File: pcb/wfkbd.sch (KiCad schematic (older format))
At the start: 124 parts, among them J1 MJ-4PP-9, P1 LED, SW1 KEY, SW10 KEY, SW11 KEY, SW12 KEY, SW13 KEY, SW14 KEY, SW15 KEY, SW16 KEY, SW17 KEY, SW18 KEY, SW19 KEY, SW2 KEY, SW20 KEY, SW21 KEY, SW22 KEY, SW23 KEY, SW24 KEY, SW25 KEY, SW26 KEY, SW27 KEY, SW28 KEY, SW29 KEY, SW3 KEY, SW30 KEY, SW31 KEY, SW32 KEY, SW33 KEY, SW34 KEY, SW35 KEY, SW4 KEY, SW5 KEY, SW6 KEY, SW7 KEY, SW8 KEY, SW9 KEY, U1 ProMicro

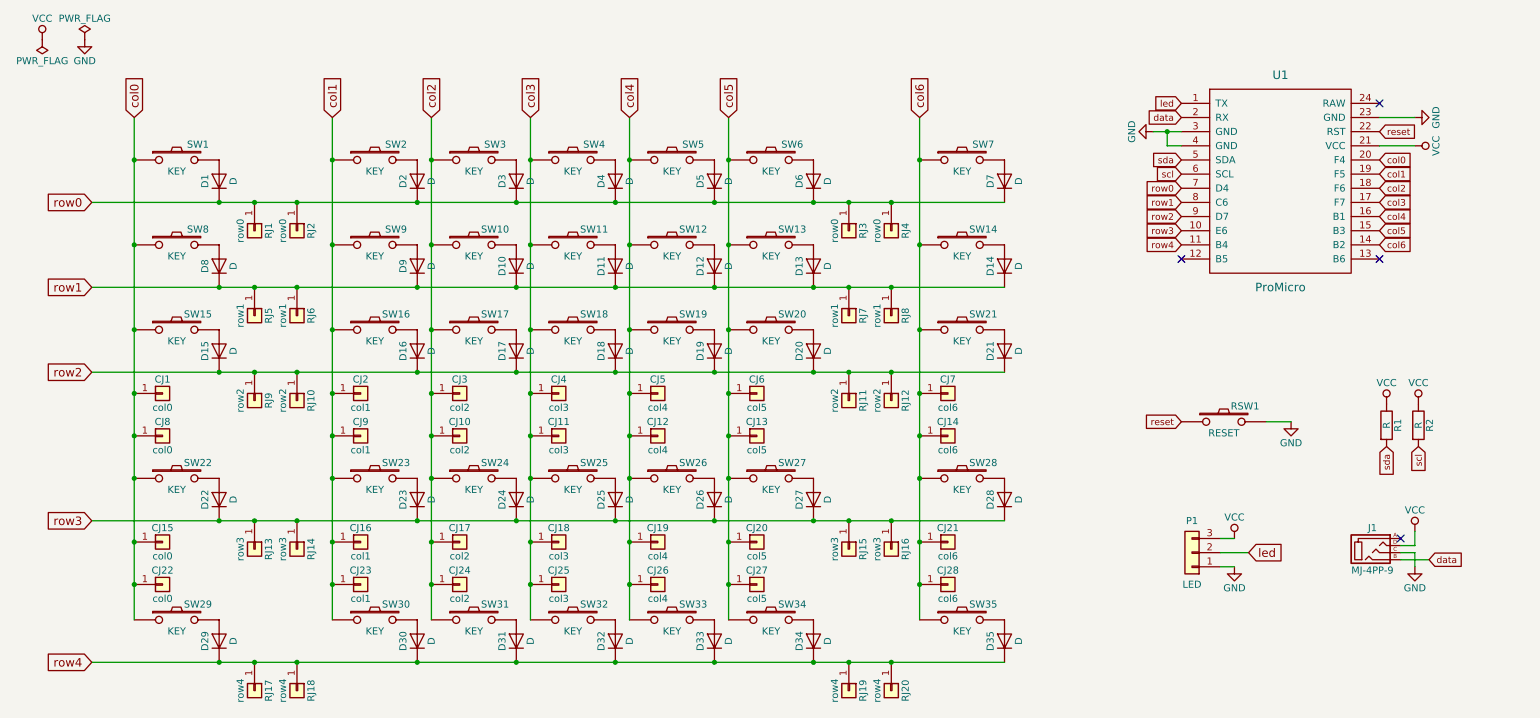
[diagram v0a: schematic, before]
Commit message: Add pcbnew files
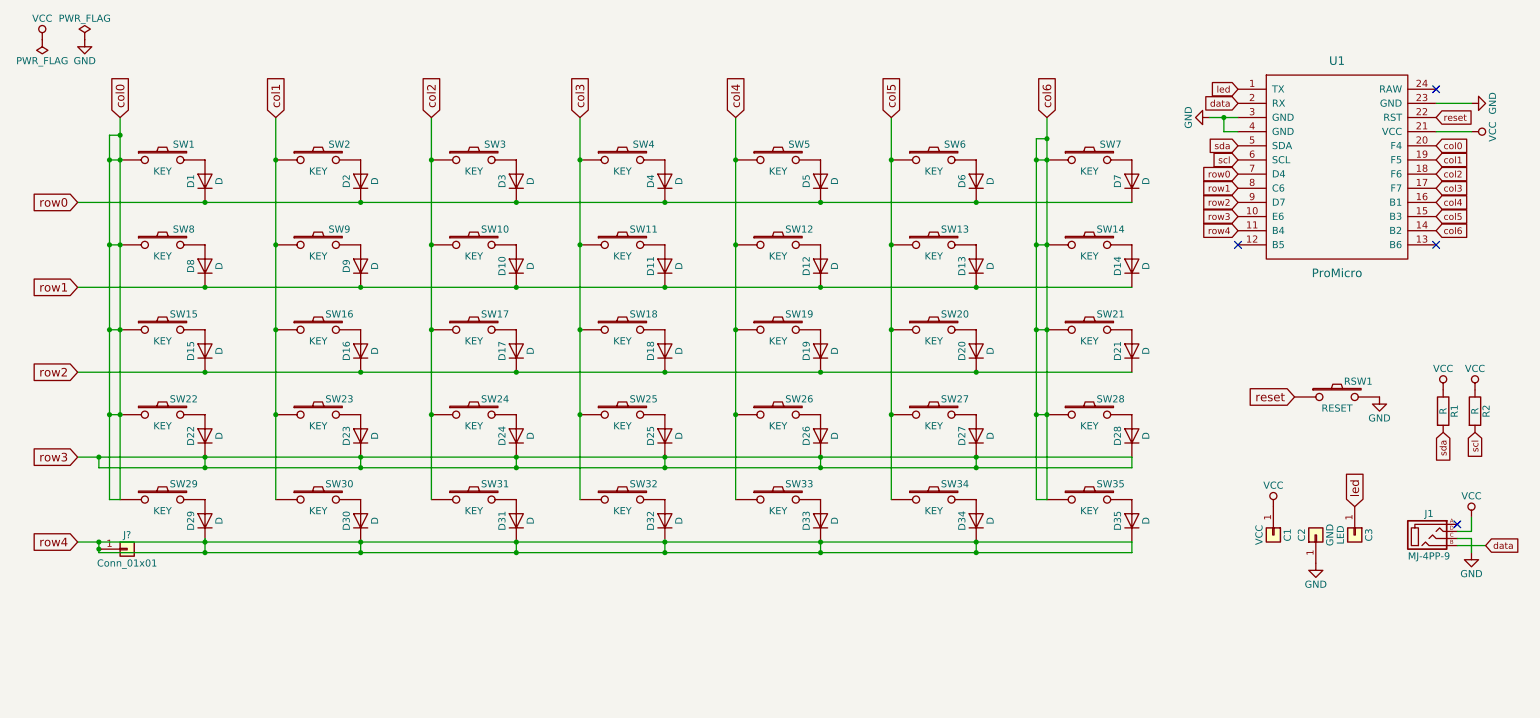
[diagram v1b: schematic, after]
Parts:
- removed CJ1, CJ15, CJ22, CJ8: col0, kbd:1pin_conn, symbol Conn_01x01
- removed CJ10, CJ17, CJ24, CJ3: col2, kbd:1pin_conn, symbol Conn_01x01
- removed CJ11, CJ18, CJ25, CJ4: col3, kbd:1pin_conn, symbol Conn_01x01
- removed CJ12, CJ19, CJ26, CJ5: col4, kbd:1pin_conn, symbol Conn_01x01
- removed CJ13, CJ20, CJ27, CJ6: col5, kbd:1pin_conn, symbol Conn_01x01
- removed CJ14, CJ21, CJ28, CJ7: col6, kbd:1pin_conn, symbol Conn_01x01
- removed CJ16, CJ2, CJ23, CJ9: col1, kbd:1pin_conn, symbol Conn_01x01
- removed P1: LED, kbd:StripLED_rev, symbol Conn_01x03
- removed RJ1, RJ2, RJ3, RJ4: row0, kbd:1pin_conn, symbol Conn_01x01
- removed RJ10, RJ11, RJ12, RJ9: row2, kbd:1pin_conn, symbol Conn_01x01
- removed RJ13, RJ14, RJ15, RJ16: row3, kbd:1pin_conn, symbol Conn_01x01
- removed RJ17, RJ18, RJ19, RJ20: row4, kbd:1pin_conn, symbol Conn_01x01
- removed RJ5, RJ6, RJ7, RJ8: row1, kbd:1pin_conn, symbol Conn_01x01
- added C1: VCC, kbd:1pin_conn, symbol Conn_01x01
- added C2: GND, kbd:1pin_conn, symbol Conn_01x01
- added C3: LED, kbd:1pin_conn, symbol Conn_01x01
- added J?: Conn_01x01, symbol Conn_01x01
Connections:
- net GND: now also C2.1 (Pin_1)
- net VCC: now also C1.1 (Pin_1)
- net led: now also C3.1 (Pin_1)
- net row4: now also J?.1 (Pin_1)
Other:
- moved on the sheet: D1, D11, D12, D13, D14, D15, D16, D18, D19, D2, D20, D21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

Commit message: Remove unused lines
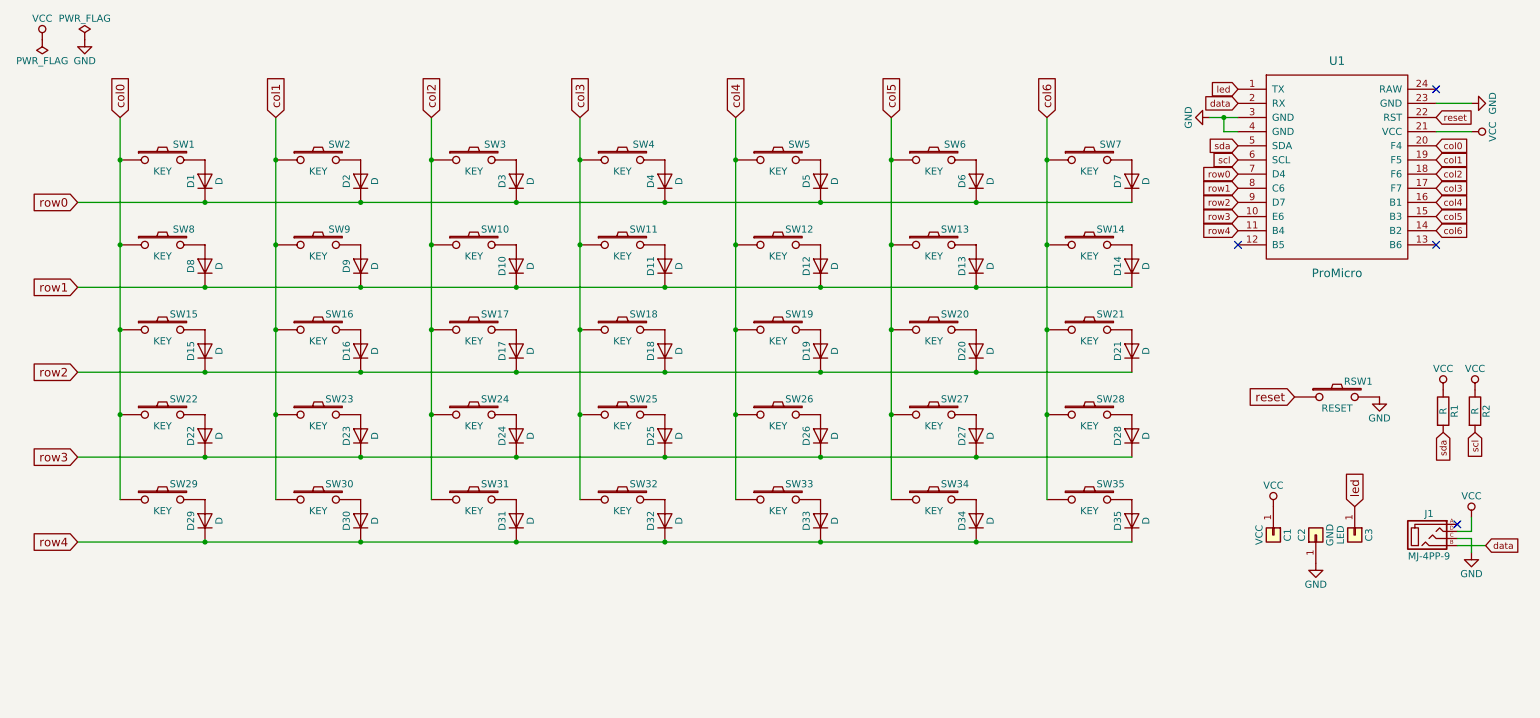
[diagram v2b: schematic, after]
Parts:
- removed J?: Conn_01x01, symbol Conn_01x01
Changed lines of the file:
@@
 	1300 1300 1300 4000
-Wire Wire Line
-	2400 1300 2400 4000
-Wire Wire Line
-	3500 1300 3500 4000
-Wire Wire Line
-	4550 1300 4550 4000
-Wire Wire Line
-	5650 1300 5650 4000
-Wire Wire Line
-	6750 1300 6750 4000
-Wire Wire Line
-	1000 1900 8450 1900
-Wire Wire Line
-	1000 2500 8450 2500
-Wire Wire Line
-	1000 3100 8450 3100
-Wire Wire Line
-	1000 3700 8450 3700
 Wire Wire Line
 	1000 4300 8450 4300
@@
 Connection ~ 1900 1900
 Wire Wire Line
-	1150 4300 1150 4375
+	1000 3700 8450 3700
 Wire Wire Line
-	1150 4375 8450 4375
+	1000 3100 8450 3100
 Wire Wire Line
-	8450 4375 8450 4300
-Connection ~ 1150 4300
+	8450 2500 1000 2500
 Wire Wire Line
-	7350 4300 7350 4375
-Connection ~ 7350 4375
+	1000 1900 8450 1900
 Wire Wire Line
-	6250 4300 6250 4375
-Connection ~ 6250 4375
+	2400 4000 2400 1300
 Wire Wire Line
-	5150 4300 5150 4375
-Connection ~ 5150 4375
+	3500 4000 3500 1300
 Wire Wire Line
-	4100 4300 4100 4375
-Connection ~ 4100 4375
+	4550 4000 4550 1300
 Wire Wire Line
-	3000 4300 3000 4375
-Connection ~ 3000 4375
+	5650 4000 5650 1300
 Wire Wire Line
-	1900 4275 1900 4375
-Connection ~ 1900 4375
-Wire Wire Line
-	1150 3700 1150 3775
-Wire Wire Line
-	1150 3775 8450 3775
-Wire Wire Line
-	8450 3775 8450 3700
-Connection ~ 1150 3700
-Wire Wire Line
-	7350 3700 7350 3775
-Connection ~ 7350 3775
-Wire Wire Line
-	6250 3700 6250 3775
-Connection ~ 6250 3775
-Wire Wire Line
-	5150 3700 5150 3775
-Connection ~ 5150 3775
-Wire Wire Line
-	4100 3700 4100 3775
-Connection ~ 4100 3775
-Wire Wire Line
-	3000 3700 3000 3775
-Connection ~ 3000 3775
-Wire Wire Line
-	1900 3700 1900 3775
-Connection ~ 1900 3775
-Wire Wire Line
-	1300 1425 1225 1425
-Wire Wire Line
-	1225 1425 1225 4000
-Wire Wire Line
-	1225 4000 1300 4000
-Connection ~ 1300 1425
-Wire Wire Line
-	1300 1600 1225 1600
-Connection ~ 1225 1600
-Wire Wire Line
-	1300 2200 1225 2200
-Connection ~ 1225 2200
-Wire Wire Line
-	1300 2800 1225 2800
-Connection ~ 1225 2800
-Wire Wire Line
-	1300 3400 1225 3400
-Connection ~ 1225 3400
-Wire Wire Line
-	7850 1450 7775 1450
-Wire Wire Line
-	7775 1450 7775 4000
-Wire Wire Line
-	7775 4000 7850 4000
-Connection ~ 7850 1450
-Wire Wire Line
-	7850 1600 7775 1600
-Connection ~ 7775 1600
-Wire Wire Line
-	7850 2200 7775 2200
-Connection ~ 7775 2200
-Wire Wire Line
-	7850 2800 7775 2800
-Connection ~ 7775 2800
-Wire Wire Line
-	7850 3400 7775 3400
-Connection ~ 7775 3400
-$Comp
-L Conn_01x01 J?
-U 1 1 5ABB6DE7
-P 1350 4350
-F 0 "J?" H 1350 4450 50  0000 C CNN
-F 1 "Conn_01x01" H 1350 4250 50  0000 C CNN
-F 2 "" H 1350 4350 50  0001 C CNN
-F 3 "" H 1350 4350 50  0001 C CNN
-	1    1350 4350
-	1    0    0    -1
-$EndComp
-Connection ~ 1150 4350
+	6750 4000 6750 1300
 $EndSCHEMATC

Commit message: To simply
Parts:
- RSW1: footprint kbd:SW_3.5x6.0_TH -> Keebio-Parts:SW_Tactile_SPST_Angled_MJTP1117
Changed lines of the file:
@@
 F 0 "RSW1" H 10050 3385 50  0000 C CNN
 F 1 "RESET" H 9900 3195 50  0000 C CNN
-F 2 "kbd:SW_3.5x6.0_TH" H 9900 3275 50  0001 C CNN
+F 2 "Keebio-Parts:SW_Tactile_SPST_Angled_MJTP1117" H 9900 3275 50  0001 C CNN
 F 3 "" H 9900 3275 50  0000 C CNN
 	1    9900 3275
